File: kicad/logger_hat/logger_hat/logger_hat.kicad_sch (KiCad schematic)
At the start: 22 parts, among them J1 CO2_sensor_conn, J10 Conn_01x04_Pin, J2 5V_sensor_conn, J3 CH4_Sensor_conn, J4 Reed_switch_conn, J5 PWM_output_1, J6 log_switch_conn, J7 PWM_output_2

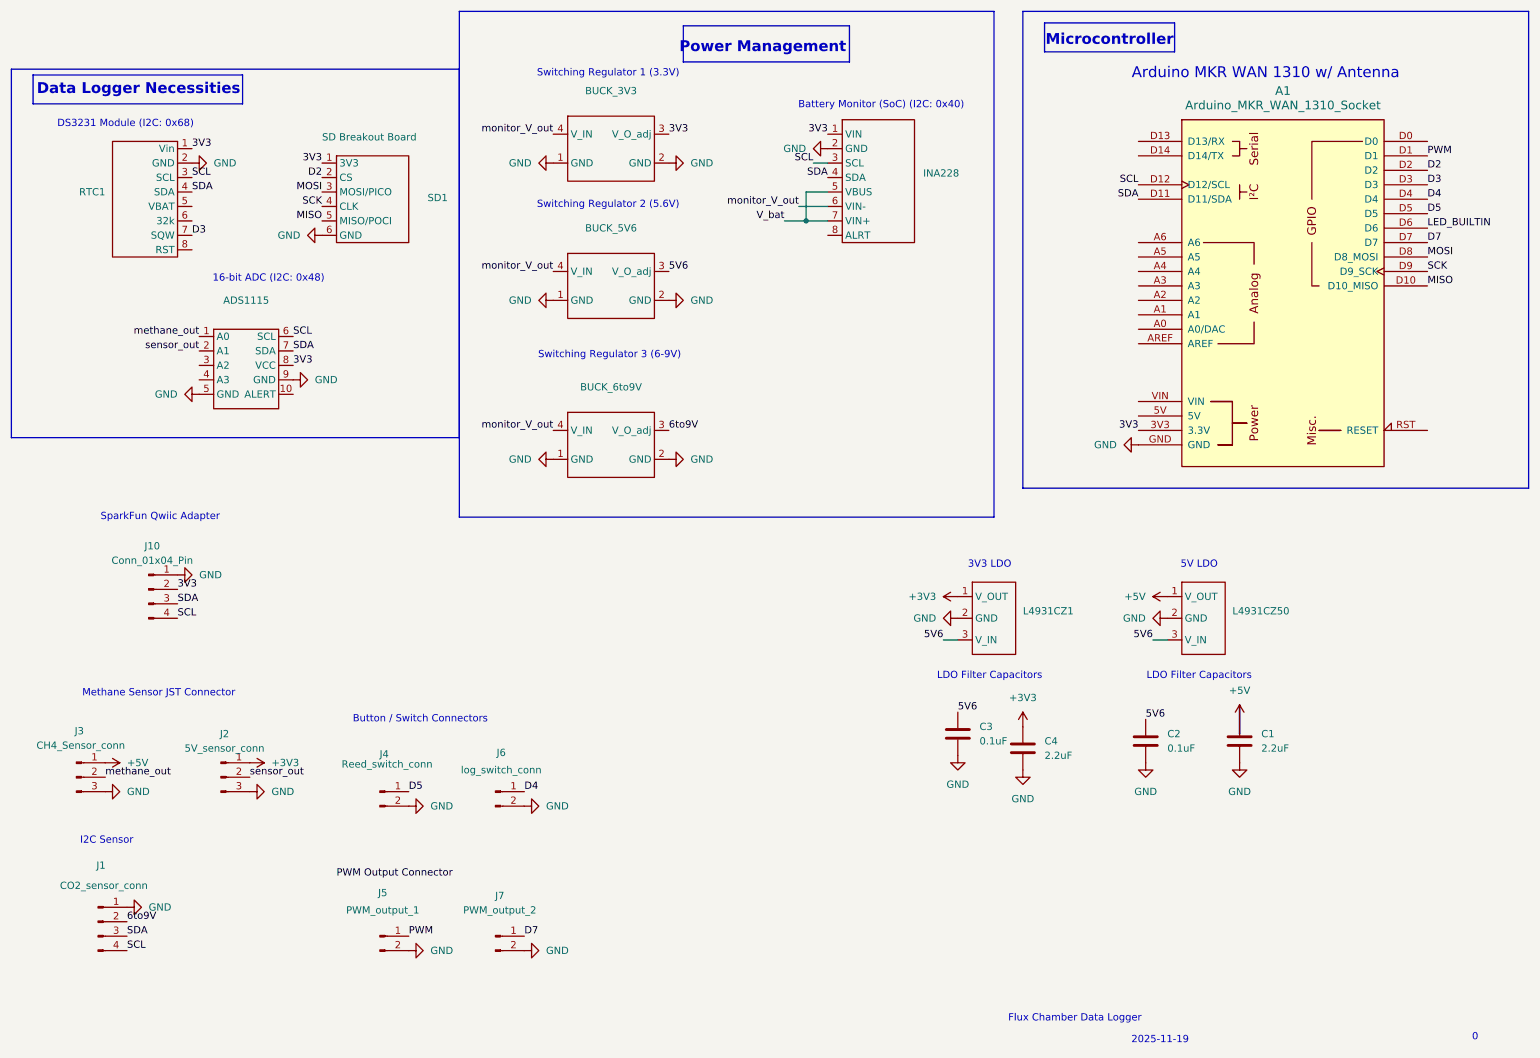
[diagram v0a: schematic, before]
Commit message: Read work log
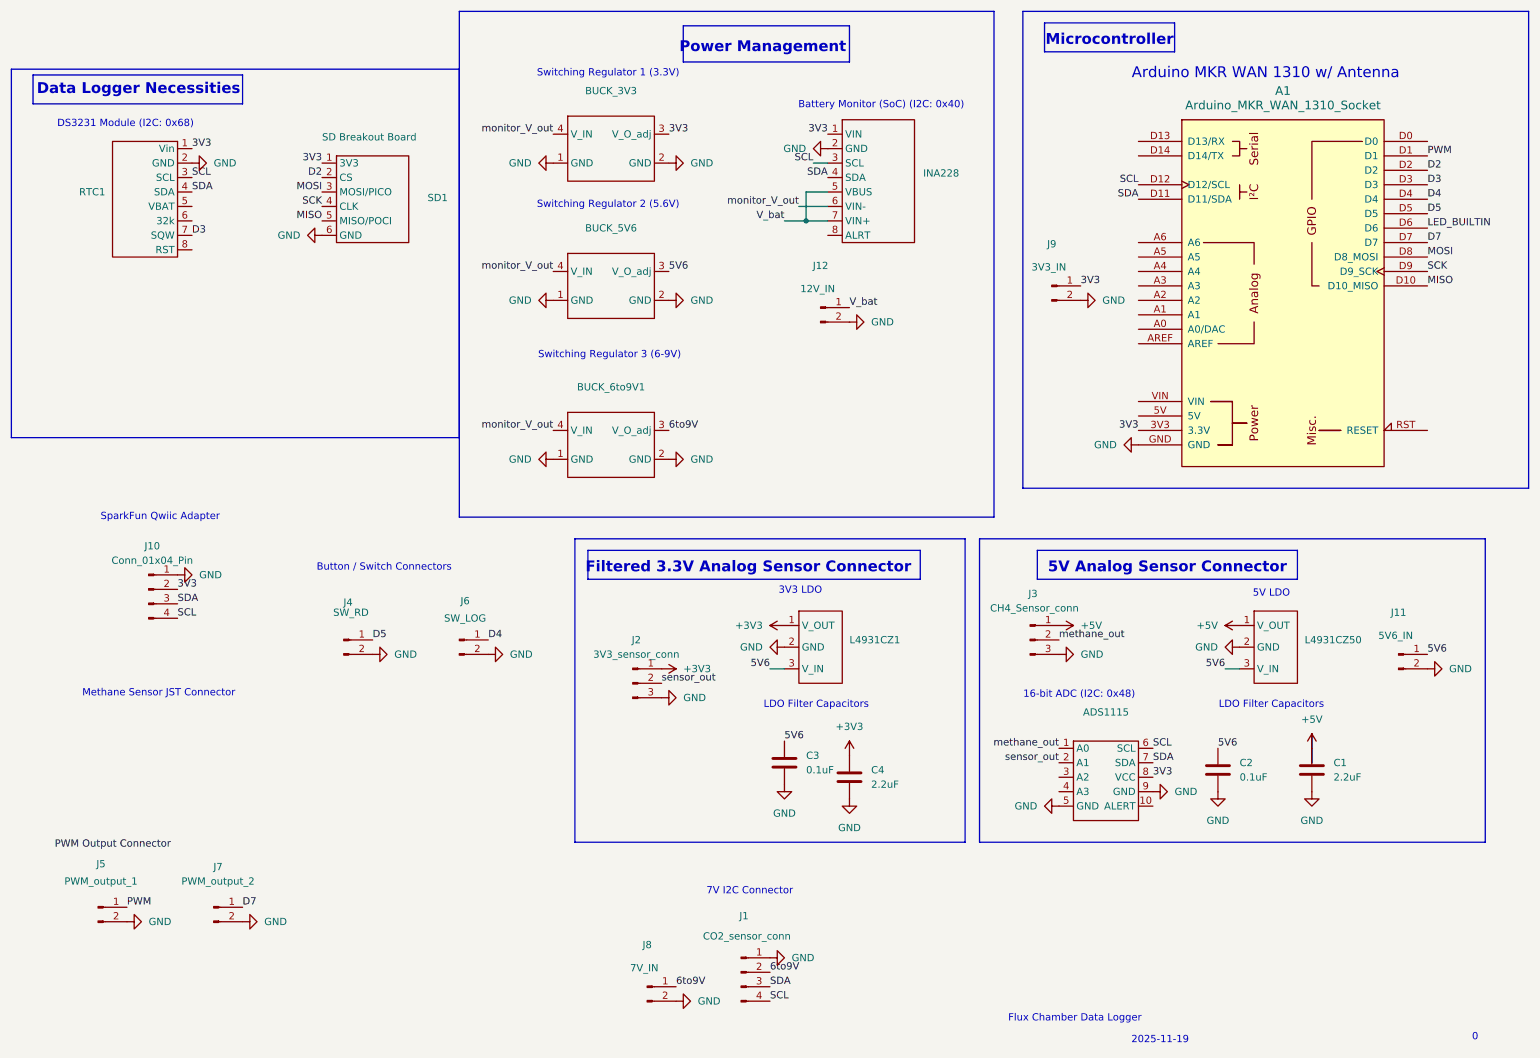
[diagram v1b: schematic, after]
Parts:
- added J11: 5V6_IN, Connector_JST:JST_XH_B2B-XH-A_1x02_P2.50mm_Vertical, symbol Connector:Conn_01x02_Pin
- added J12: 12V_IN, Connector_JST:JST_XH_B2B-XH-A_1x02_P2.50mm_Vertical, symbol Connector:Conn_01x02_Pin
- added J8: 7V_IN, Connector_JST:JST_XH_B2B-XH-A_1x02_P2.50mm_Vertical, symbol Connector:Conn_01x02_Pin
- added J9: 3V3_IN, Connector_JST:JST_XH_B2B-XH-A_1x02_P2.50mm_Vertical, symbol Connector:Conn_01x02_Pin
- J2: value 5V_sensor_conn -> 3V3_sensor_conn
- J4: value Reed_switch_conn -> SW_RD
- J6: value log_switch_conn -> SW_LOG
- L4931CZ1, L4931CZ50: footprint Package_TO_SOT_THT:TO-92_Inline -> Package_TO_SOT_THT:TO-92_HandSolder
- renumbered BUCK_6to9V to BUCK_6to9V1
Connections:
- net 3V3: now also J9.1 (Pin_1)
- net 5V6: now also J11.1 (Pin_1)
- net 6to9V: now also J8.1 (Pin_1)
- net GND: now also J11.2 (Pin_2), J12.2 (Pin_2), J8.2 (Pin_2), J9.2 (Pin_2)
- net V_bat: now also J12.1 (Pin_1)
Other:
- note added: "5V Analog Sensor Connector"
- note added: "7V I2C Connector"
- note added: "Filtered 3.3V Analog Sensor Connector"
- note removed: "I2C Sensor"
- moved on the sheet: ADS1115, C1, C2, C3, C4, J1, J2, J3, J4, J5, J6, J7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
